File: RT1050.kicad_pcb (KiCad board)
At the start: 4 copper layers, 88 x 94.5 mm, 110 parts, among them IC1 IS42S16160J-6BLI, IC2 S26KL512SDABHV020, J1 Conn_01x04_Pin, J10 Conn_01x06_Pin, J13 Conn_02x04_Counter_Clockwise, J14 Conn_02x04_Counter_Clockwise, J2 Conn_01x04_Pin, J3 Conn_01x20, J4 Conn_01x05_Pin, J5 USB_C_Receptacle_USB2.0, J6 Conn_01x02, J7 Conn_01x02, J8 Conn_Coaxial_Small, J9 Conn_01x04_Pin, SW1 SW_DIP_x02, U1 MIMXRT1052CVJ5B, U10 TPS22921YZPR, U11 TPS22921YZPR, U12 CY15B064J-SXET, U2 DP83TC813SRHFRQ1, U3 MMC5983MA, U4 BMI088, U5 RFM98W-433S2, U6 TCAN334, U7 PRTR5V0U2X, U8 XC6206P332PR-G, U9 MCP23009-E/MG, Y1 DSC1001BI5-024.0000, Y2 830107834801

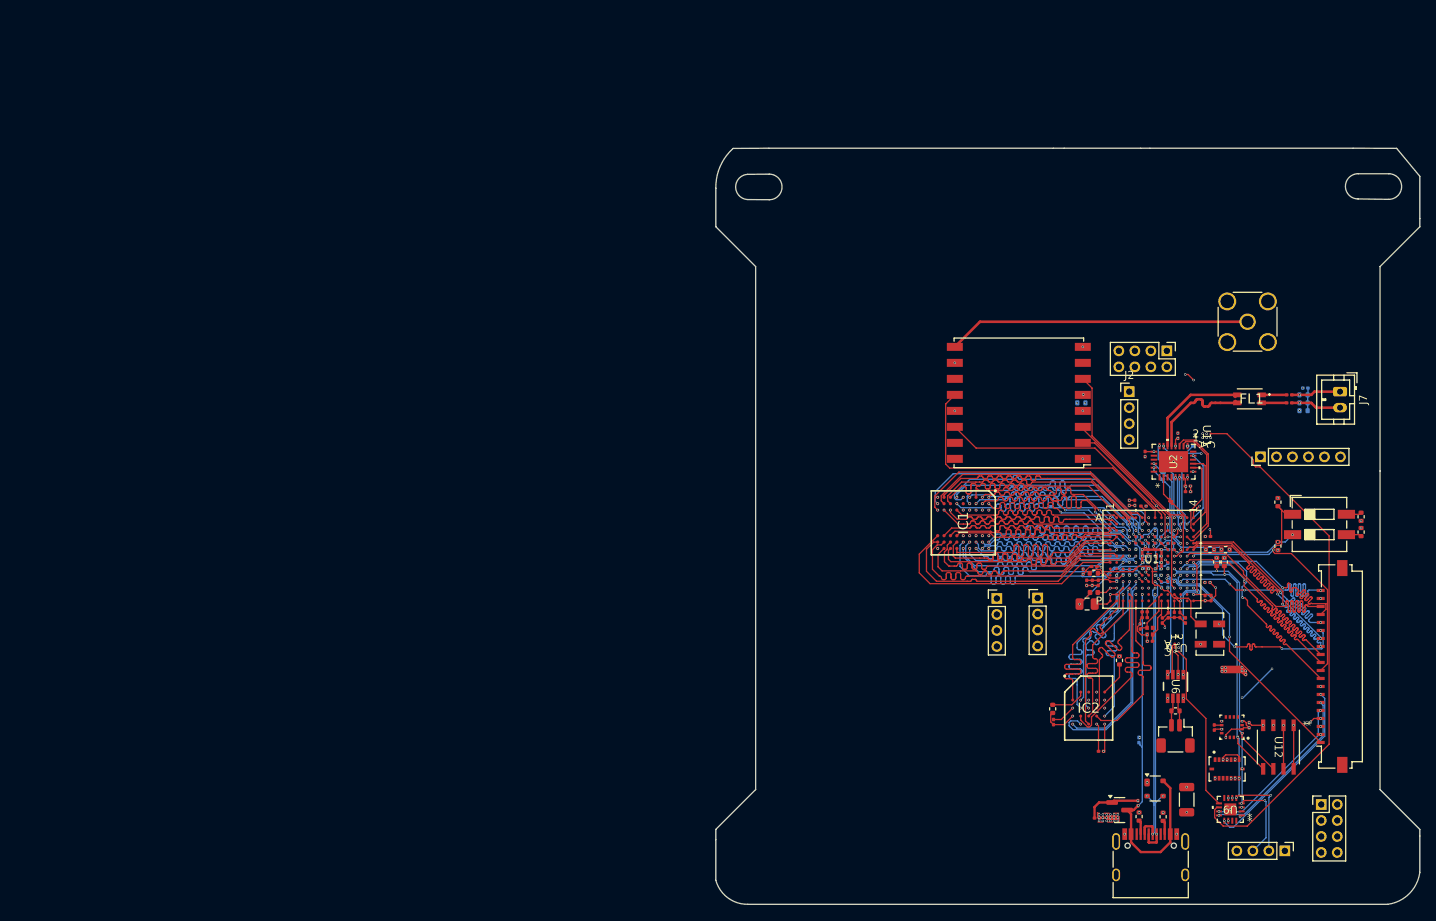
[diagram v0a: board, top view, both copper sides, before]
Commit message: updated schem pdf
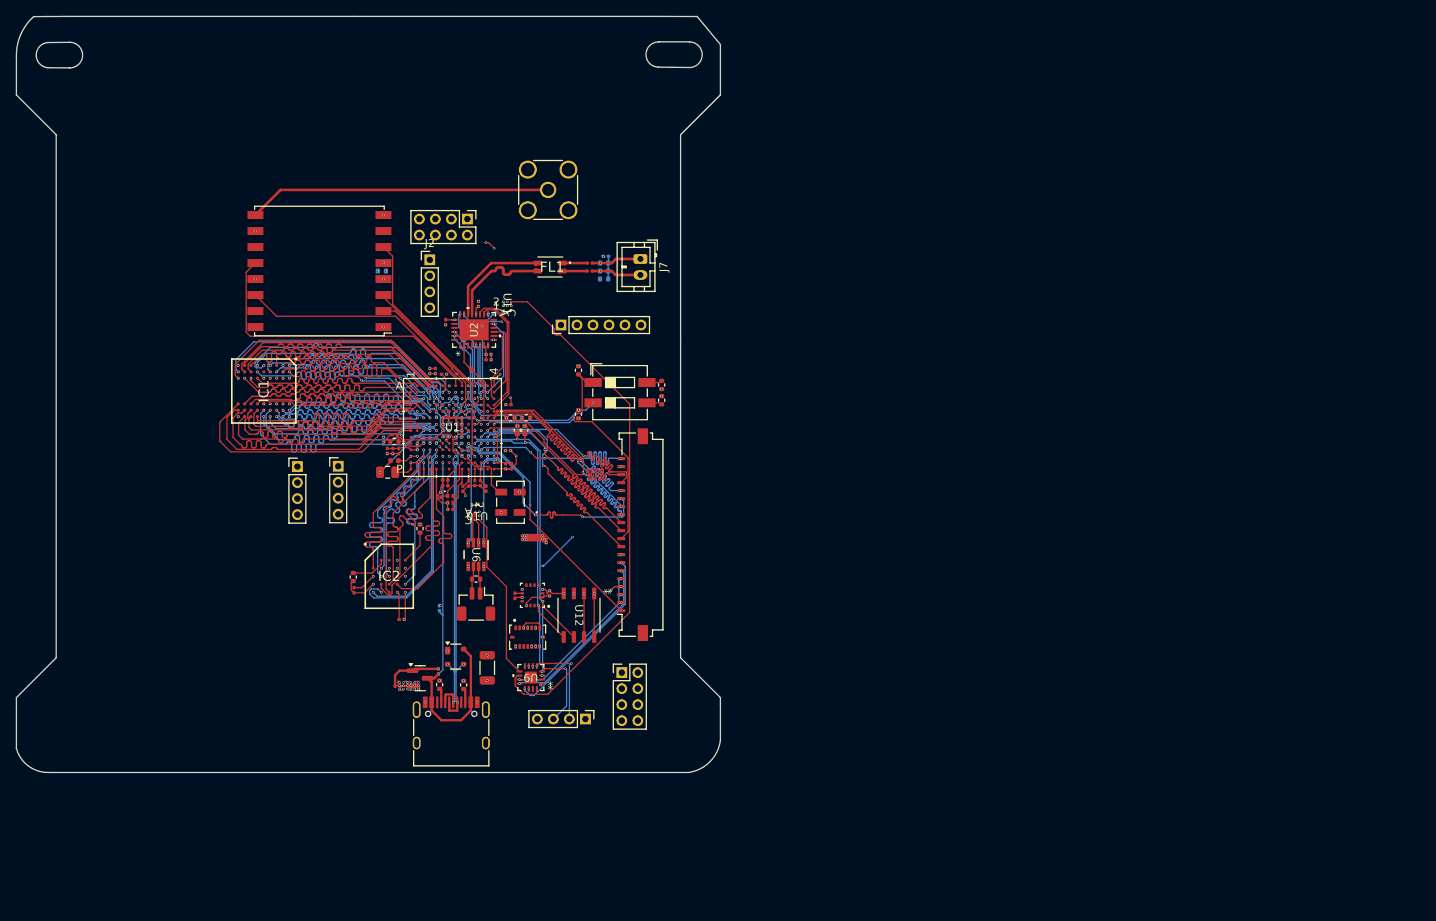
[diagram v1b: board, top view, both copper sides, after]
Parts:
- moved J7 89.0 mm to (101.5, 53.3)
- moved C10 89.0 mm to (85.0, 71.5)
- moved C11 89.0 mm to (77.1, 80.9)
- moved C12 89.0 mm to (77.1, 81.6)
- moved C13 89.0 mm to (84.7, 79.2)
- moved C14 89.0 mm to (85.4, 79.2)
- moved C15 89.0 mm to (80.0, 77.5)
- moved C17 89.0 mm to (81.5, 81.3)
- moved C22 89.0 mm to (77.8, 84.6)
- moved C27 89.0 mm to (73.6, 76.7)
- moved C28 89.0 mm to (69.8, 77.3)
- moved C30 89.0 mm to (69.9, 79.9)
- moved C31 89.0 mm to (74.4, 75.9)
- moved C34 89.0 mm to (76.4, 96.9)
- moved C35 89.0 mm to (76.4, 71.5)
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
